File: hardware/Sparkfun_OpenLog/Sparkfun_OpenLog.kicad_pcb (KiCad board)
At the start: 2 copper layers, 15.2 x 19 mm, 26 parts, among them Q1 16MHZ, U1 ATMEGA328P_TQFP, U2 3.3V MIC5205, U3 microSD Socket

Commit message: Updated Schematic
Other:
- rule pad_to_mask_clearance: 0 -> 0.05
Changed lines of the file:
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@@
 		(0 "F.Cu" signal)
 		(2 "B.Cu" signal)
-		(9 "F.Adhes" user "F.Adhesive")
-		(11 "B.Adhes" user "B.Adhesive")
 		(13 "F.Paste" user)
 		(15 "B.Paste" user)
@@
 		(1 "F.Mask" user)
 		(3 "B.Mask" user)
-		(17 "Dwgs.User" user "User.Drawings")
-		(19 "Cmts.User" user "User.Comments")
-		(21 "Eco1.User" user "User.Eco1")
-		(23 "Eco2.User" user "User.Eco2")
+		(17 "Dwgs.User" user "Measures")
+		(19 "Cmts.User" user "V-score")
+		(21 "Eco1.User" user "Fab.Info")
+		(23 "Eco2.User" user "License.Info")
 		(25 "Edge.Cuts" user)
 		(27 "Margin" user)
 		(31 "F.CrtYd" user "F.Courtyard")
 		(29 "B.CrtYd" user "B.Courtyard")
-		(35 "F.Fab" user)
-		(33 "B.Fab" user)
-		(39 "User.1" user)
-		(41 "User.2" user)
-		(43 "User.3" user)
-		(45 "User.4" user)
+		(35 "F.Fab" user "F.Outlines")
+		(33 "B.Fab" user "B.Outlines")
+		(39 "User.1" user "Milling")
+		(41 "User.2" user "Design.Info")
+		(43 "User.3" user "Board.Properties")
+		(45 "User.4" user "Selective.Solder")
+		(47 "User.5" user "Enclosure.Info")
 	)
 	(setup
-		(pad_to_mask_clearance 0)
+		(stackup
+			(layer "F.SilkS"
+				(type "Top Silk Screen")
+				(color "#FFFFFFFF")
+			)
+			(layer "F.Paste"
+				(type "Top Solder Paste")
+			)
+			(layer "F.Mask"
+				(type "Top Solder Mask")
+				(color "#E0311DD4")
+				(thickness 0.01)
+			)
+			(layer "F.Cu"
+				(type "copper")
+				(thickness 0.035)
+			)
+			(layer "dielectric 1"
+				(type "core")
+				(thickness 1.51)
+				(material "FR4")
+				(epsilon_r 4.5)
+				(loss_tangent 0.02)
+			)
+			(layer "B.Cu"
+				(type "copper")
+				(thickness 0.035)
+			)
+			(layer "B.Mask"
+				(type "Bottom Solder Mask")
+				(color "#E0311DD4")
+				(thickness 0.01)
+			)
+			(layer "B.Paste"
+				(type "Bottom Solder Paste")
+			)
+			(layer "B.SilkS"
+				(type "Bottom Silk Screen")
+				(color "#FFFFFFFF")
+			)
+			(copper_finish "None")
+			(dielectric_constraints no)
+		)
+		(pad_to_mask_clearance 0.05)
 		(allow_soldermask_bridges_in_footprints no)
 		(tenting front back)

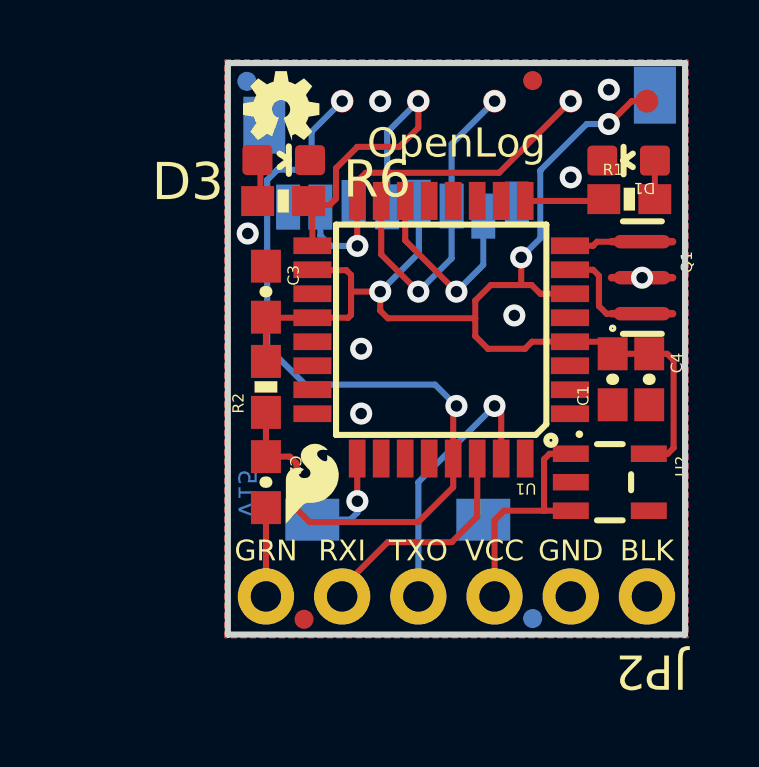
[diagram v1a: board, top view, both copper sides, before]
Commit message: Updated PCB File
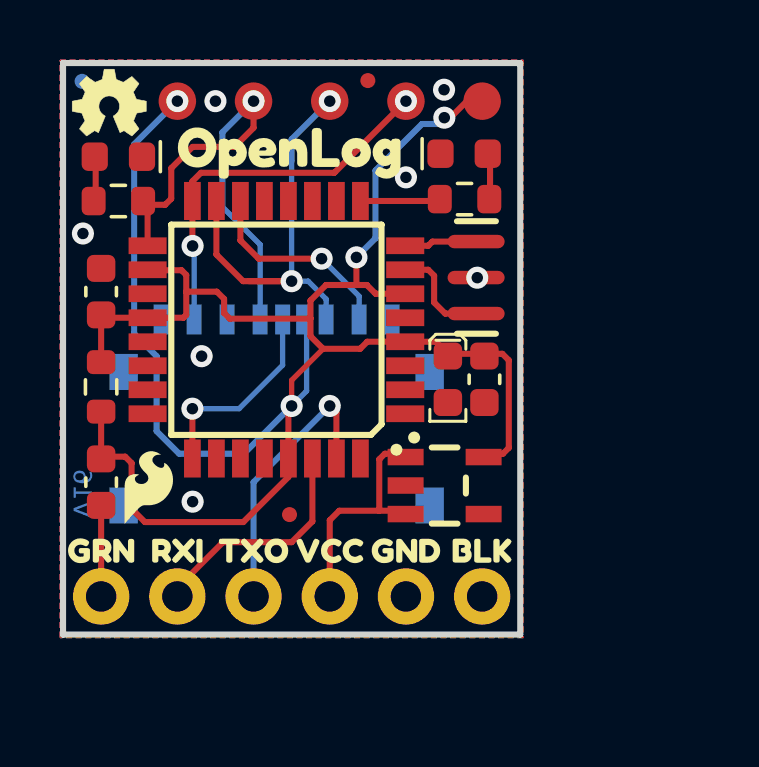
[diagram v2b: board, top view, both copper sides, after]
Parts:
- removed FRAME1: FRAME-LETTER, CREATIVE_COMMONS
- removed JP2: , 1X06_NO_SILK
- removed LOGO1: SFE_LOGO_FLAME.1_INCH, SFE_LOGO_FLAME_.1
- removed LOGO2: OSHW-LOGOMINI, OSHW-LOGO-MINI
- removed Q1: 16MHZ, RESONATOR-SMD
- removed U3: microSD Socket, MICROSD_1_1
- added G***: Flame, SparkFun-Aesthetic:SparkFun_Flame_2.5mm, F.Cu at (138.2, 109.6)
- added G***: LOGO, SparkFun-Aesthetic:SparkFun_Logo_10mm, B.Cu at (143.1, 101.0)
- added G1: OSHW_Logo, SparkFun-Aesthetic:Creative_Commons_License, F.Cu at (13.6, 7.12)
- added J1: Conn_01x06, SparkFun-Connector:1x06_P2.54mm, F.Cu at (149.4, 113.3)
- added J2: microSD_Friction, SparkFun-Connector:microSD_Friction_Fit_Common, B.Cu at (142.5, 108.0)
- added Ref**: Val**, SparkFun-Aesthetic:OSHW_Logo_2.5mm, F.Cu at (136.9, 96.9)
- added Y1: Resonator, SparkFun-Clock:Resonator_SMD_3.2x1.3mm, F.Cu at (149.2, 102.6)
- added kibuzzard-69F12217: G***, kibuzzard-69F12217, F.Cu at (136.7, 111.7)
- added kibuzzard-69F12217: G***, kibuzzard-69F12217, B.Cu at (136.7, 111.7)
- added kibuzzard-69F1223A: G***, kibuzzard-69F1223A, F.Cu at (139.2, 111.7)
- added kibuzzard-69F1223A: G***, kibuzzard-69F1223A, B.Cu at (139.2, 111.7)
- added kibuzzard-69F1224C: G***, kibuzzard-69F1224C, F.Cu at (141.7, 111.7)
- added kibuzzard-69F1224C: G***, kibuzzard-69F1224C, B.Cu at (141.7, 111.8)
- added kibuzzard-69F1225D: G***, kibuzzard-69F1225D, F.Cu at (144.3, 111.7)
- added kibuzzard-69F1225D: G***, kibuzzard-69F1225D, B.Cu at (144.3, 111.7)
- added kibuzzard-69F1226C: G***, kibuzzard-69F1226C, F.Cu at (146.8, 111.7)
- added kibuzzard-69F1226C: G***, kibuzzard-69F1226C, B.Cu at (146.8, 111.7)
- added kibuzzard-69F12278: G***, kibuzzard-69F12278, F.Cu at (149.4, 111.7)
- added kibuzzard-69F12278: G***, kibuzzard-69F12278, B.Cu at (149.3, 111.7)
- added kibuzzard-69F12315: G***, kibuzzard-69F12315, F.Cu at (142.9, 98.5)
- C1: footprint 0603-POL -> SparkFun-Capacitor:C_0603_1608Metric_Polar
- C2, C3, C4: footprint 0603-CAP -> SparkFun-Capacitor:C_0603_1608Metric
- D1: value BLUE -> Blue; footprint LED-0603 -> SparkFun-LED:LED_0603_1608Metric_Blue
- D3: value GREEN -> Green; footprint LED-0603 -> SparkFun-LED:LED_0603_1608Metric_Green
- FID1, FID2, FID3, FID4: value FIDUCIALUFIDUCIAL -> Fiducial_0.5mm; footprint MICRO-FIDUCIAL -> SparkFun-Aesthetic:Fiducial_0.5mm_Mask1mm
- R1: value 1K -> 1k; footprint 0603-RES -> SparkFun-Resistor:R_0603_1608Metric
- R2: value 10K -> 10k; footprint 0603-RES -> SparkFun-Resistor:R_0603_1608Metric
- R6: footprint 0603-RES -> SparkFun-Resistor:R_0603_1608Metric
- TP1, TP2, TP3, TP4, TP5: value TEST-POINT3 -> 1.25mm; footprint PAD.03X.03 -> SparkFun-Connector:TestPoint-1.25mm
- U1: value ATMEGA328P_TQFP -> ATmega328P; footprint TQFP32-08 -> SparkFun-Semiconductor-Standard:TQFP-32_7x7mm_P0.8mm
- U2: value 3.3V MIC5205 -> RT9080-3.3; footprint SOT23-5 -> SparkFun-Semiconductor-Standard:SOT23-5
- moved D3 5.51 mm to (137.2, 98.6), turned to 180 degrees
- moved U2 5.51 mm to (148.1, 109.6), turned to 0 degrees
- moved C1 5.49 mm to (148.2, 106.0), turned to -90 degrees
- moved C2 5.49 mm to (136.7, 109.4)
- moved C3 5.49 mm to (136.7, 103.1)
- moved C4 5.49 mm to (149.4, 106.0)
- moved FID1 5.49 mm to (145.5, 96.1)
- moved FID4 5.49 mm to (136.0, 96.1)
- moved R1 5.49 mm to (148.8, 100.0)
- moved R2 5.49 mm to (136.7, 106.3)
- moved R6 5.49 mm to (137.2, 100.1)
- moved TP1 5.49 mm to (149.4, 96.7)
- moved TP2 5.49 mm to (146.8, 96.7)
- moved TP3 5.49 mm to (144.3, 96.7)
- moved TP4 5.49 mm to (141.7, 96.7)
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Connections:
- net N$4 renamed STAT
- net RAW renamed VRAW
- C2 pad 1: RST -> ~{RST}
- C3 pad 2: 3.3V -> ~{RST}
- C4 pad 1: 3.3V -> ~{RST}
- R1 pad 2: N$3 -> Net-(D1-A)
- R2 pad 1: RST -> ~{RST}
- R2 pad 2: 3.3V -> ~{RST}
- R6 pad 2: N$7 -> Net-(D3-A)
- U1 pad 1: (no net) -> unconnected-(U1-PD3-Pad1)
- U1 pad 10: (no net) -> unconnected-(U1-PD6-Pad10)
- U1 pad 11: (no net) -> unconnected-(U1-PD7-Pad11)
- U1 pad 12: (no net) -> unconnected-(U1-PB0-Pad12)
- U1 pad 13: (no net) -> unconnected-(U1-PB1-Pad13)
- U1 pad 14: CS -> ~{CS}
- U1 pad 15: MOSI -> PICO
- U1 pad 16: MISO -> POCI
- U1 pad 18: 3.3V -> ~{RST}
- U1 pad 19: (no net) -> unconnected-(U1-ADC6-Pad19)
- U1 pad 2: (no net) -> unconnected-(U1-PD4-Pad2)
- U1 pad 20: 3.3V -> ~{RST}
- U1 pad 22: (no net) -> unconnected-(U1-ADC7-Pad22)
- U1 pad 23: (no net) -> unconnected-(U1-PC0-Pad23)
- U1 pad 24: (no net) -> unconnected-(U1-PC1-Pad24)
- U1 pad 26: (no net) -> unconnected-(U1-PC3-Pad26)
- U1 pad 27: (no net) -> unconnected-(U1-PC4-Pad27)
- U1 pad 28: (no net) -> unconnected-(U1-PC5-Pad28)
- U1 pad 29: RST -> ~{RST}
- U1 pad 32: (no net) -> unconnected-(U1-PD2-Pad32)
- U1 pad 4: 3.3V -> ~{RST}
- U1 pad 6: 3.3V -> ~{RST}
- U2 pad 4: (no net) -> unconnected-(U2-NC-Pad4)
- U2 pad 5: 3.3V -> ~{RST}
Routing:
- net ~{RST}: track 0.00 -> 71.5 mm, vias 0 -> 4
- net 3.3V: track 39.7 -> 0.00 mm, vias 3 -> 0
- net RST: track 29.5 -> 0.00 mm, vias 2 -> 0
- net PICO: track 0.00 -> 14.7 mm, vias 0 -> 2
- net POCI: track 0.00 -> 12.9 mm, vias 0 -> 2
- net MISO: track 12.7 -> 0.00 mm, vias 2 -> 0
- net MOSI: track 11.3 -> 0.00 mm, vias 2 -> 0
- net ~{CS}: track 0.00 -> 6.82 mm, vias 0 -> 1
- net CS: track 6.62 -> 0.00 mm, vias 1 -> 0
- net SCK: track 11.6 -> 15.8 mm
- net CD: track 3.41 -> 6.79 mm
- net Net-(D3-A): track 0.00 -> 1.63 mm
- net N$7: track 1.63 -> 0.00 mm
- net Net-(D1-A): track 0.00 -> 1.29 mm
- net N$3: track 1.29 -> 0.00 mm
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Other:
- board text added: "V16"
- board text removed: "+"
- board text removed: "-"
- board text removed: "BLK"
- board text removed: "GND"
- board text removed: "GRN"
- board text removed: "N. Seidle"
- board text removed: "OpenLog"
- board text removed: "RXI"
- board text removed: "Revised by: Patrick Alberts, Pete Lewis"
- board text removed: "TXO"
- board text removed: "V15"
- board text removed: "VCC"
